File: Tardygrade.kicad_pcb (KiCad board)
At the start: 2 copper layers, 50 x 50 mm, 23 parts, among them J1 Conn_01x03, J2 Conn_01x03, J3 Conn_01x03, J4 Conn_01x03, J5 Conn_01x03_Male, U1 MCP1642B, U2 HUZZAH32, U3 Tinypico, U4 HallSwitch, U5 HallSwitch, U6 HallSwitch, U7 HallSwitch, X1 XpansionHeader

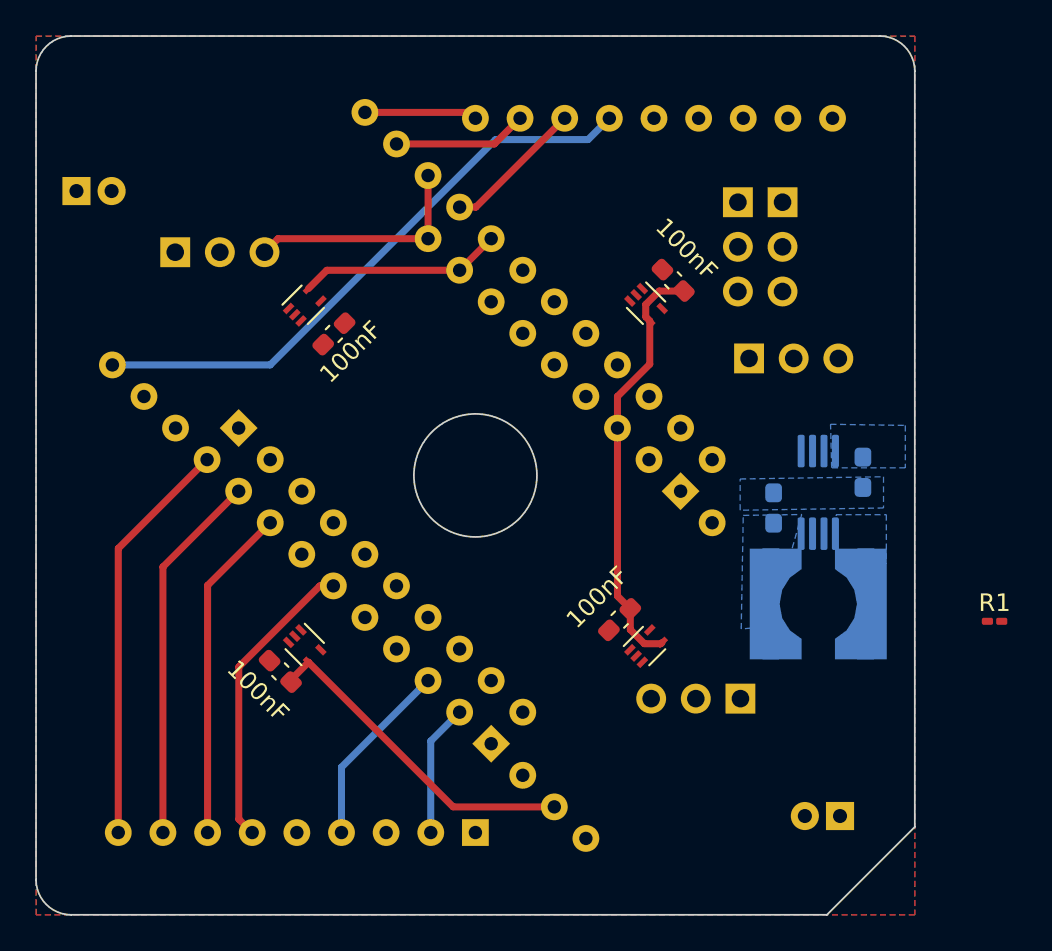
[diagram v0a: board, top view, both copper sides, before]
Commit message: v.04 update3
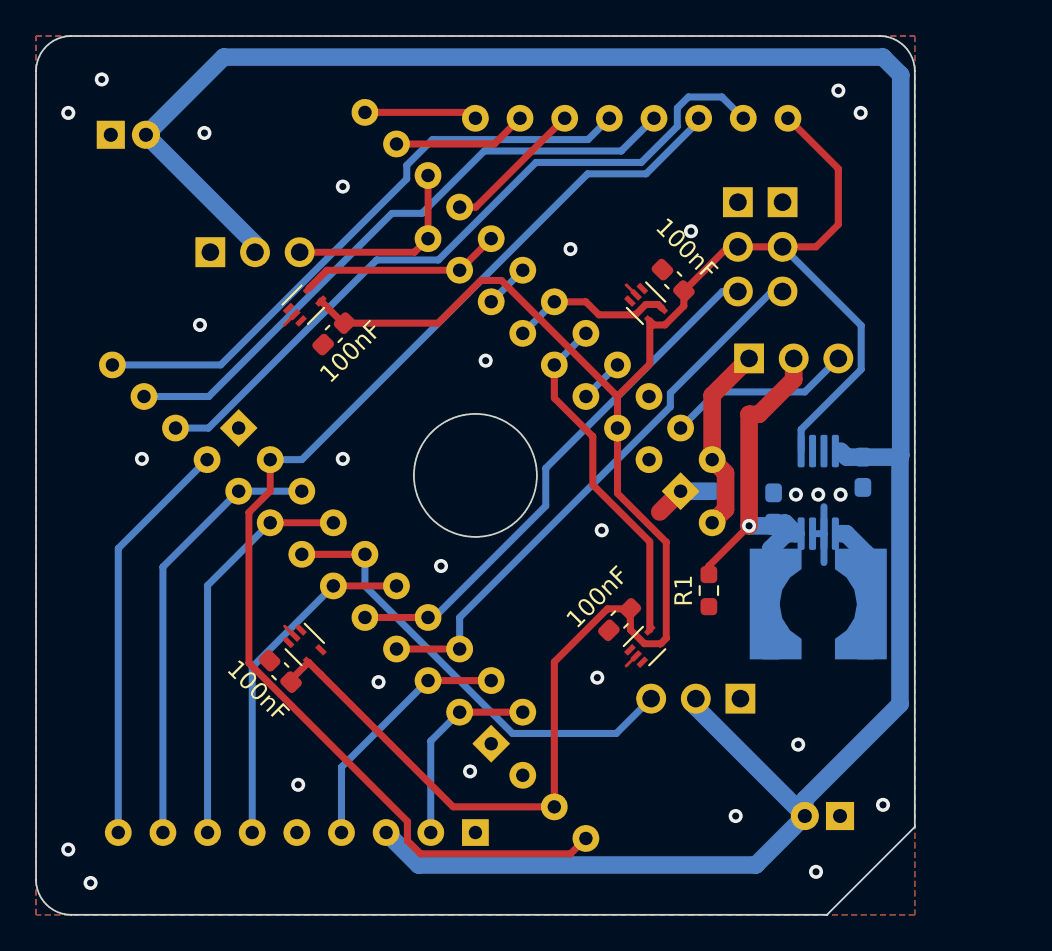
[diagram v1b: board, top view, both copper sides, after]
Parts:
- R1: footprint Resistor_SMD:R_0201_0603Metric_Pad0.64x0.40mm_HandSolder -> Resistor_SMD:R_0603_1608Metric_Pad0.98x0.95mm_HandSolder
- moved R1 16.3 mm to (113.3, 106.6), turned to 90 degrees
- moved C3 3.75 mm to (81.3, 80.6)
- moved J1 2.00 mm to (90.0, 87.3)
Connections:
- U1 pad 1: BOOST_EN -> 3V3_Rail
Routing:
- net 5V_Rail: track 0.00 -> 137.4 mm
- net 3V3_Rail: track 43.3 -> 113.4 mm
- net Reset: track 0.00 -> 69.3 mm
- net RX: track 0.00 -> 41.2 mm
- net TX: track 0.00 -> 35.6 mm
- net LidarFront: track 0.00 -> 31.9 mm
- net LidarRear: track 0.16 -> 30.3 mm
- net ServoRear: track 0.00 -> 26.0 mm
- net VBAT_Rail: track 0.00 -> 22.5 mm, vias 0 -> 1
- net HallRight: track 0.00 -> 19.9 mm
- net VBAT: track 0.00 -> 10.9 mm
- net GND: track 0.00 -> 10.7 mm, vias 0 -> 27
- net EN: track 0.00 -> 10.6 mm
- net HallRear: track 0.00 -> 9.33 mm
- net Net-(L1-Pad1): track 0.00 -> 4.77 mm
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- removed copper zone on B.Cu, net 5V_Rail
- removed copper zone on B.Cu, net Net-(L1-Pad1)
- removed copper zone on B.Cu, net VBAT_Rail

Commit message: v0.4 update 4
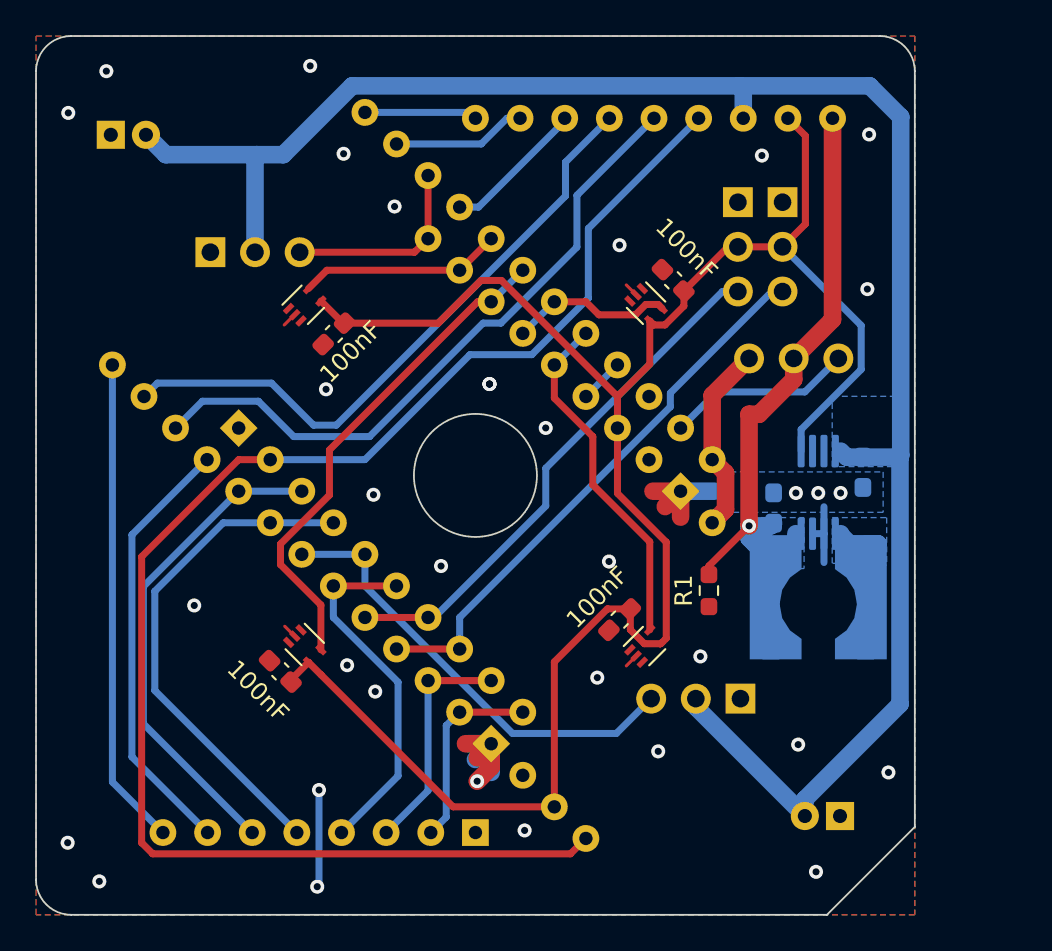
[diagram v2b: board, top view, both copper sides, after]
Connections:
- X1 pad 1: 3V3_Rail -> VBAT_Rail
- X1 pad 12: 5V_Rail -> DAC1
- X1 pad 13: DAC1 -> GPIO36
- X1 pad 14: VBAT_Drain -> SCK
- X1 pad 15: GPIO36 -> MOSI
- X1 pad 16: SCK -> MISO
- X1 pad 17: MOSI -> GPIO21
- X1 pad 2: RX -> 3V3_Rail
- X1 pad 3: Reset -> 5V_Rail
- X1 pad 4: TX -> Reset
- X1 pad 6: GPIO21 -> TX
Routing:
- net 5V_Rail: track 137.4 -> 108.6 mm
- net HallFront: track 2.54 -> 28.7 mm
- net GND: track 10.7 -> 28.1 mm, vias 27 -> 34
- net Reset: track 69.3 -> 86.5 mm
- net VBAT_Rail: track 22.5 -> 39.6 mm
- net GPIO21: track 34.5 -> 27.8 mm
- net SCK: track 22.7 -> 28.9 mm
- net Net-(L1-Pad1): track 4.77 -> 9.64 mm
- net RX: track 41.2 -> 37.9 mm
- net MOSI: track 24.8 -> 27.8 mm
- net 3V3_Rail: track 113.4 -> 110.7 mm
- net MISO: track 23.3 -> 24.8 mm
- net DAC1: track 14.3 -> 13.2 mm
- net GPIO36: track 19.5 -> 20.5 mm
- net TX: track 35.6 -> 36.1 mm
- added copper zone on B.Cu, net 5V_Rail
- added copper zone on B.Cu, net Net-(L1-Pad1)
- added copper zone on B.Cu, net VBAT_Rail
